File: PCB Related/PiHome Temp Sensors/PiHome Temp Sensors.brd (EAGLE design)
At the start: 71.1 x 50.8 mm, 13 parts, among them M1 WIRELESS-NRF24L01, U1 DS18B20

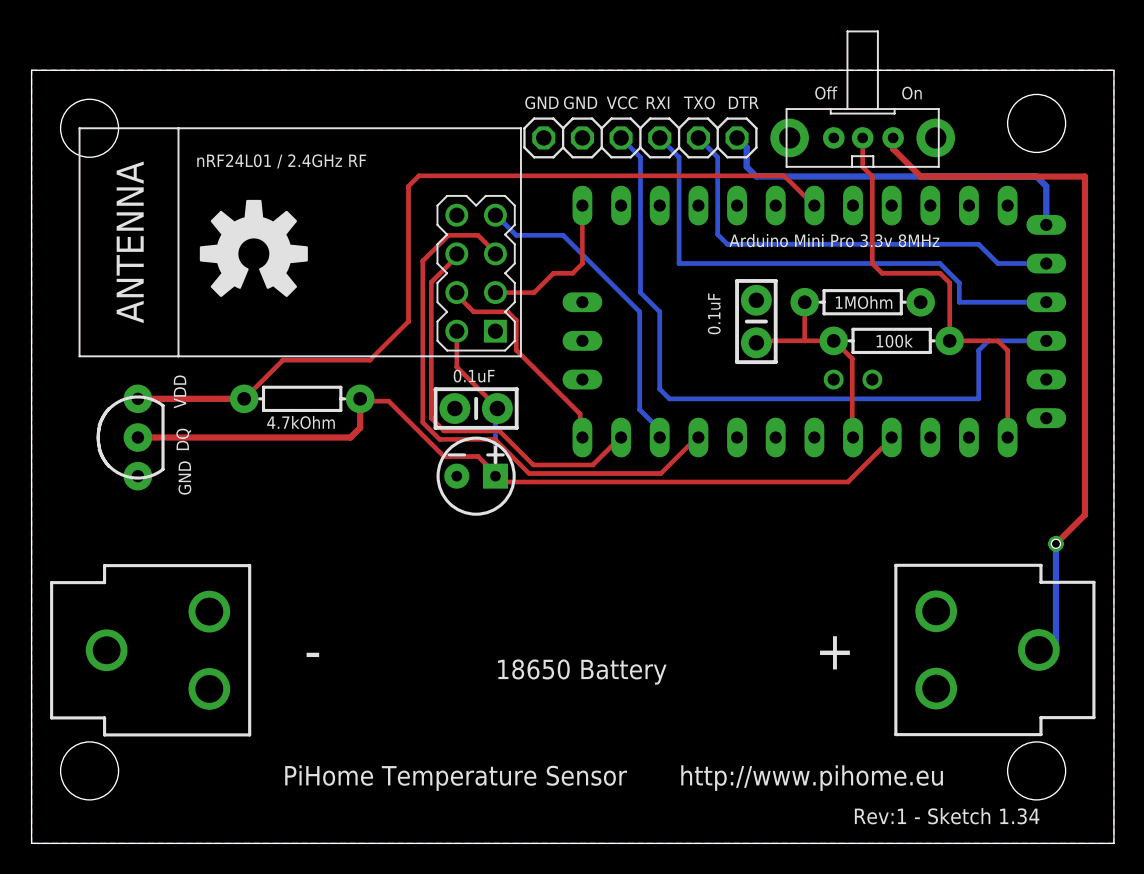
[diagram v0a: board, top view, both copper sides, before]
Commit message: Improved PCB Design
Improved PCB Design
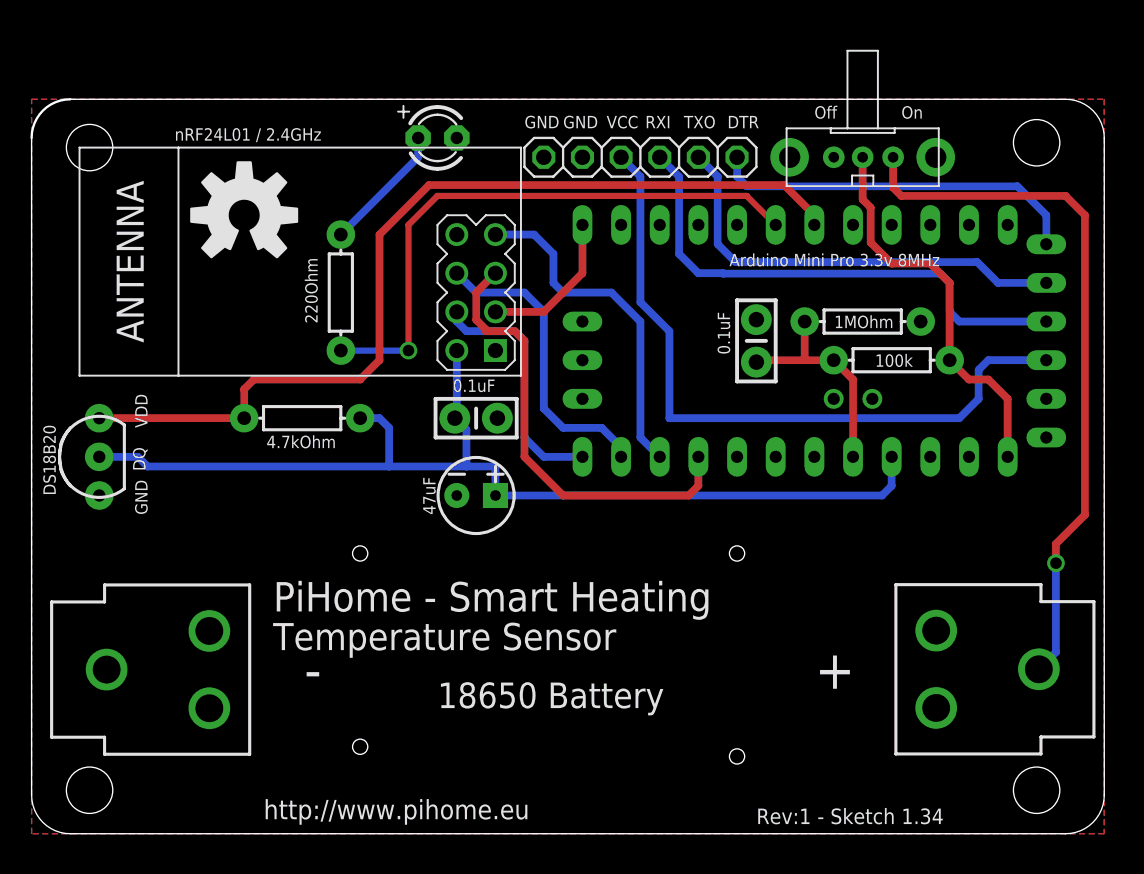
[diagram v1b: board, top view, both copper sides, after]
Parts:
- added LED1: (no value), adafruit:LED3MM
- added R5: 220Ohm, SparkFun-Resistors:AXIAL-0.3
- moved U1 2.84 mm to (4.45, 25.4)
- moved LOGO1 2.62 mm to (14.0, 41.3)
- moved M1 1.27 mm to (17.8, 38.7)
- moved R1 1.27 mm to (56.5, 31.8)
- moved R2 1.27 mm to (54.6, 34.3)
- moved BAT1 1.27 mm to (35.6, 11.4)
- moved C3 1.27 mm to (29.2, 22.9)
- moved R3 1.27 mm to (17.8, 27.9)
- moved C2 1.27 mm to (47.6, 33.0)
- moved JP1 1.27 mm to (40.0, 45.1)
- moved S1 1.27 mm to (54.6, 45.1)
- moved U$1 1.27 mm to (57.8, 35.6)
- moved C1 0.63 mm to (29.2, 27.9), turned to 0 degrees
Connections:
- new net D4: R5.P$1, U$1.D4
- new net N$1: LED1.A, R5.P$2
- net GND: now also LED1.K
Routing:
- net D4: track 0.00 -> 38.4 mm, vias 0 -> 1
- net N$1: track 0.00 -> 8.45 mm, vias 1 -> 0
- net SCK: track 37.1 -> 29.7 mm
- net MOSI: track 26.0 -> 19.9 mm
- net VDD: track 56.7 -> 60.7 mm
- net 3.3V: track 66.0 -> 69.1 mm
- net CSN: track 14.3 -> 16.3 mm
- net VCC: track 27.7 -> 25.9 mm
- net MISO: track 21.1 -> 22.4 mm
- net RXI: track 34.7 -> 34.0 mm
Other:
- board size 71.1 x 50.8 mm -> 70.5 x 48.3 mm
- board text added: "DS18B20"
- board text added: "PiHome - Smart Heating"
- board text added: "Temperature Sensor"
- board text added: "nRF24L01 / 2.4GHz"
- board text removed: "PiHome Temperature Sensor"
- board text removed: "nRF24L01 / 2.4GHz RF"
